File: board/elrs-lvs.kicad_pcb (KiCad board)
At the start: 4 copper layers, 46 x 22 mm, 85 parts, among them J1 PWM, J10 CF/Prog, J12 Balance, J13 U.FL, J2 PWM, J3 PWM, J4 PWM, J5 PWM, J6 PWM, J7 PWM, J8 PWM, J9 Little Tower, SW1 SW_SPST, SW2 SW_SPST, U1 ESP32-PICO-V3, U2 SX1281, U3 TPSM82901SISR, U4 2450FM07D0034T, Y1 52Mhz TCXO

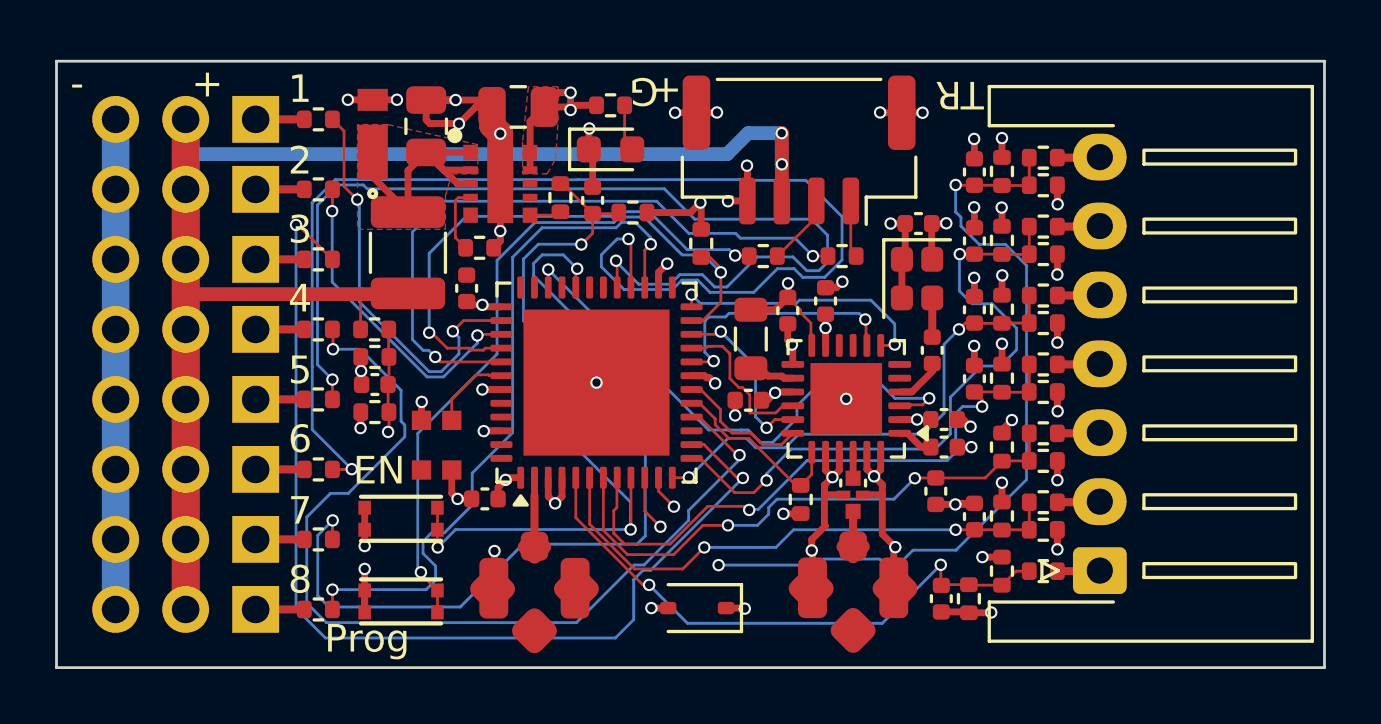
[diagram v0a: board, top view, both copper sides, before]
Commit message: more cleanup
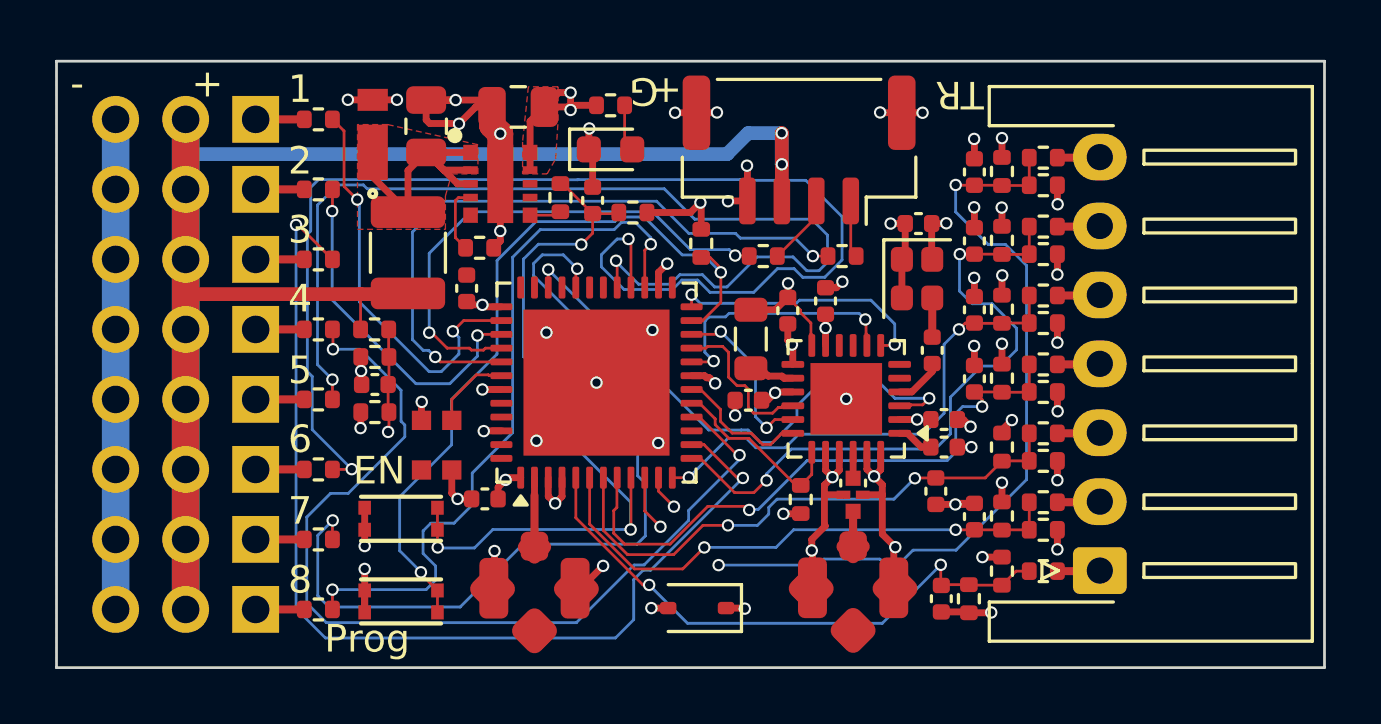
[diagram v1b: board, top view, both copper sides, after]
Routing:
- net GND: track 260.9 -> 265.5 mm, vias 43 -> 48
- net /PWM2: track 11.7 -> 12.6 mm
- net /BOOT: track 27.3 -> 27.8 mm
- net /PWM6: track 46.3 -> 46.8 mm
